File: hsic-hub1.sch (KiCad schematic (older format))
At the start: 17 parts

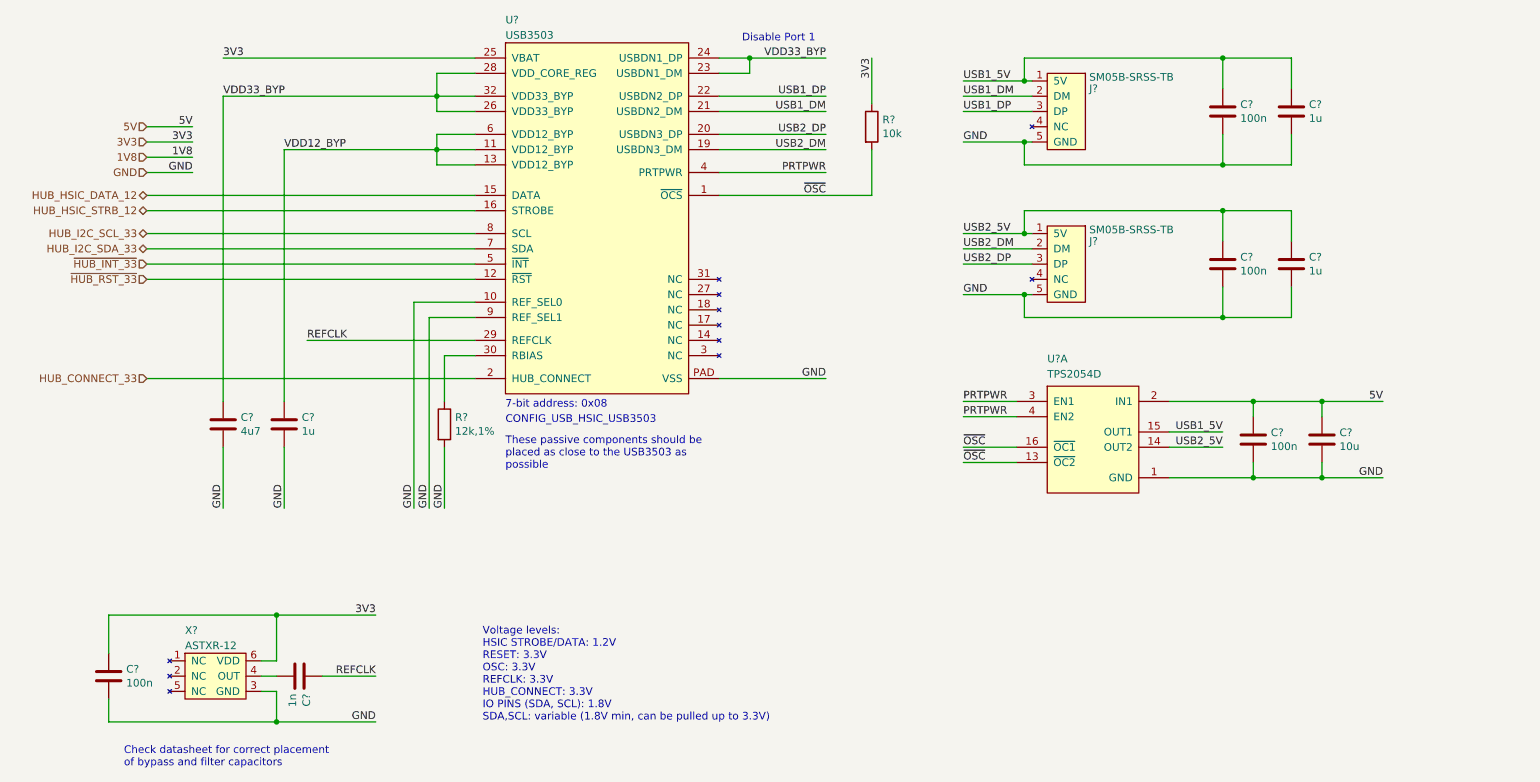
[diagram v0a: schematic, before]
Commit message: Minor fixes.
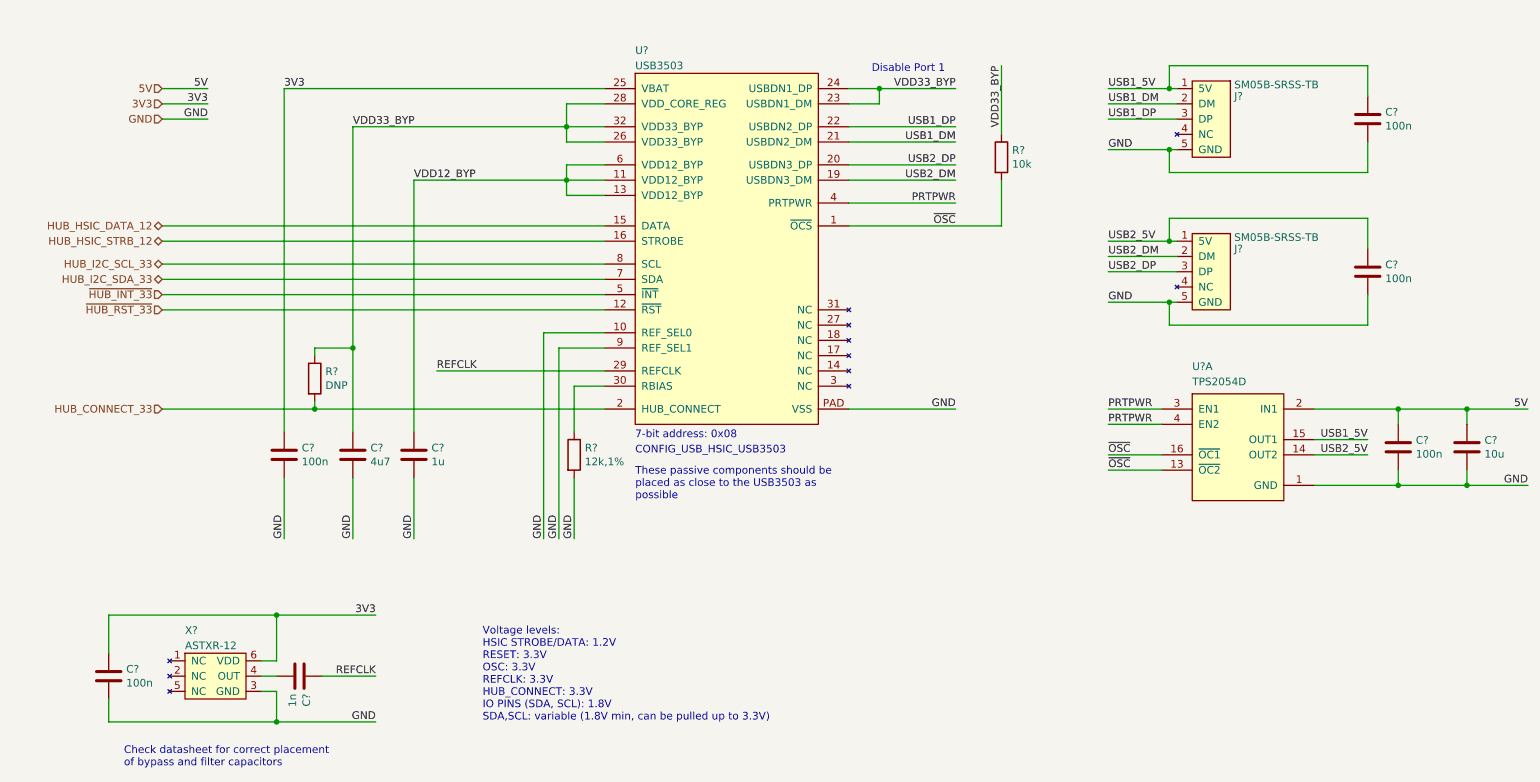
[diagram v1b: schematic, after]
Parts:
- removed C? (x2): 100n, Capacitor_SMD:C_0805_2012Metric_Pad1.15x1.40mm_HandSolder, symbol Drone:CAP
- removed C? (x2): 1u, Capacitor_SMD:C_0805_2012Metric_Pad1.15x1.40mm_HandSolder, symbol Drone:CAP
- removed J? (x2): SM05B-SRSS-TB, Drone:SM05B-SRSS-TB, symbol Drone:SM05B-SRSS-TB
- added C? (x3): 100n, Capacitor_SMD:C_0805_2012Metric_Pad1.15x1.40mm_HandSolder, symbol Drone:CAP
- added J? (x2): SM05B-SRSS-TB, Drone:SM05B-SRSS-TB, symbol Drone:SM05B-SRSS-TB
- added R?: DNP, Resistor_SMD:R_0805_2012Metric_Pad1.15x1.40mm_HandSolder, symbol Drone:RES
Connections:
- net 3V3: now also C?.1; no longer R?.1
- net GND: now also C?.2, C?.2, C?.2, J?.5 (GND), J?.5 (GND)
- net HUB_CONNECT_33: now also R?.2
- net USB1_5V: now also C?.1, J?.1 (5V)
- net USB1_DM: now also J?.2 (DM)
- net USB1_DP: now also J?.3 (DP)
- net USB2_5V: now also C?.1, J?.1 (5V)
- net USB2_DM: now also J?.2 (DM)
- net USB2_DP: now also J?.3 (DP)
- net VDD33_BYP: now also R?.1, R?.1
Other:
- moved on the sheet: C?, R?, U?, U?A
